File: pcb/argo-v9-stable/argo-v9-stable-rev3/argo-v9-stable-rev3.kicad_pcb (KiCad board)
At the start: 2 copper layers, 94.8 x 67.2 mm, 91 parts, among them IC1 MP2672GD, J1 Sparkfun_NEO-N9M-SMA, J2 USB4125-GF-A, J3 LED_power_button_RGB_LED, K1 PRL3-5V-DC-1A, Q2 BSD840N, SW1 POW, U1 orange_pi_zero_2w_2GB, U2 MAX11612, U3 CH221K, U5 SHT45-ADB1B, U6 RA-01, U7 TXS0102DCT

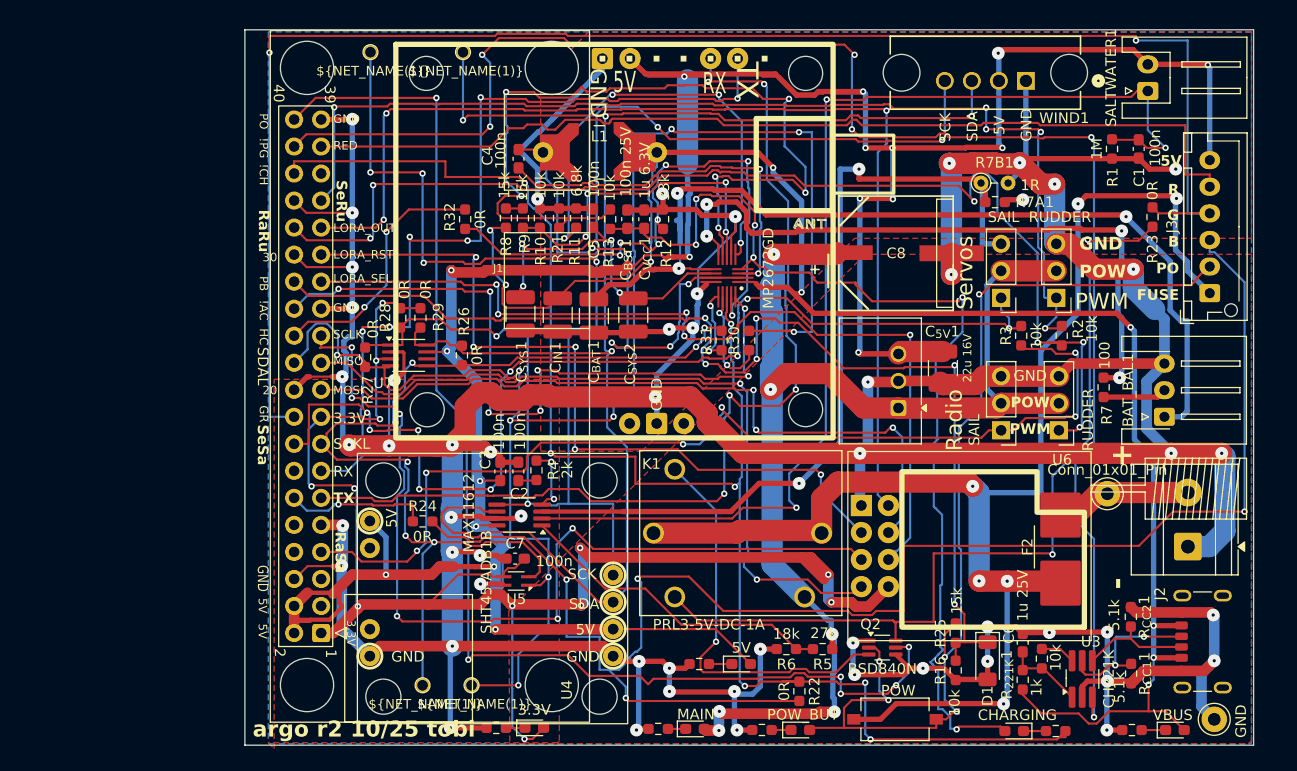
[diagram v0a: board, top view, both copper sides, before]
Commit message: argo pcb rev3 almost complete
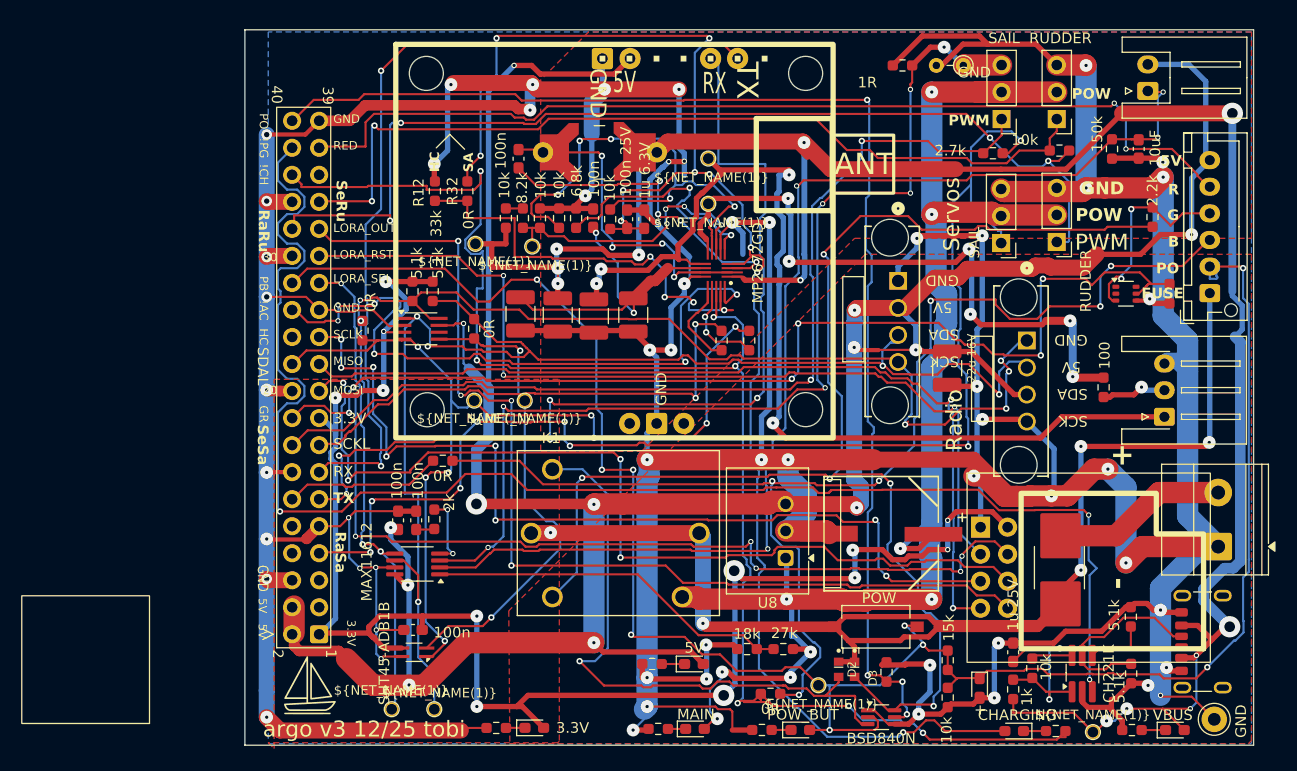
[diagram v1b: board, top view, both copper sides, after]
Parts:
- removed 5VREG1: Traco TSR1-2450E, Converter_DCDC:Converter_DCDC_TRACO_TSR1-xxxxE_THT
- removed BAT2: Conn_01x01_Pin, Connector_Pin:Pin_D1.0mm_L10.0mm_LooseFit
- added D2: TS4148_RCG, Argo footprint Library:DIO_TS4148_RCG, F.Cu at (113.0, 88.5)
- added D3: TS4148_RCG, Argo footprint Library:DIO_TS4148_RCG, F.Cu at (114.5, 88.5)
- added G***: LOGO, Argo footprint Library:argo-sailboat-icon, F.Cu at (63.2, 90.0)
- added Q1: BSD840N, Package_TO_SOT_SMD:SOT-363_SC-70-6, F.Cu at (140.0, 53.2)
- added R33: 10k, Resistor_SMD:R_0603_1608Metric_Pad0.98x0.95mm_HandSolder, F.Cu at (117.5, 88.8)
- added R34: 10k, Resistor_SMD:R_0603_1608Metric_Pad0.98x0.95mm_HandSolder, F.Cu at (144.1, 53.2)
- added TP10: TestPoint_Probe_autonamed, Argo footprint Library:TestPoint_scope_probe_autonamed, F.Cu at (84.2, 48.8)
- added TP11: TestPoint_Probe_autonamed, Argo footprint Library:TestPoint_scope_probe_autonamed, F.Cu at (136.9, 94.4)
- added TP5: TestPoint_Probe_autonamed, Argo footprint Library:TestPoint_scope_probe_autonamed, F.Cu at (78.9, 48.5)
- added TP6: TestPoint_Probe_autonamed, Argo footprint Library:TestPoint_scope_probe_autonamed, F.Cu at (111.1, 90.0)
- added TP8: TestPoint_Probe_autonamed, Argo footprint Library:TestPoint_scope_probe_autonamed, F.Cu at (100.8, 44.8)
- added TP9: TestPoint_Probe_autonamed, Argo footprint Library:TestPoint_scope_probe_autonamed, F.Cu at (100.8, 40.5)
- added U8: TSR_1-2450, Argo footprint Library:Converter_DCDC_TRACO_TSR1-xxxxE_THT, F.Cu at (108.0, 78.0)
- C1: value 100n -> 10uF
- D1: footprint Diode_SMD:D_MiniMELF -> Argo footprint Library:D_0603_1608Metric_hand_solder
- J3: footprint Connector_JST:JST_XH_B6B-XH-AM_1x06_P2.50mm_Vertical -> Argo footprint Library:JST_XH_B6B-XH-AM_1x06_P2.50mm_Vertical
- K1: footprint PRL3-5V-DC-1A:RELAY_PRL3-5V-DC-1A -> Argo footprint Library:RELAY_PRL3-5V-DC-1A
- Q2: footprint Package_TO_SOT_SMD:SOT-363_SC-70-6 -> Argo footprint Library:SOT-363_SC-70-6-handsolder
- R1: value 1M -> 150k
- R19: value 0R -> 1k
- R23: value 0R -> 2.2k
- R28, R29: value 0R -> 5.1k
- R3: value 10k -> 2.7k
- R8: value 15k -> 10k
- R9: value 15k -> 8.2k
- TP1: value SDA -> TestPoint_Probe_autonamed; footprint Argo footprint Library:TestPoint_scope_probe -> Argo footprint Library:TestPoint_scope_probe_autonamed
- TP2: value SCK -> TestPoint_Probe_autonamed; footprint Argo footprint Library:TestPoint_scope_probe -> Argo footprint Library:TestPoint_scope_probe_autonamed
- TP3: value SDAL -> TestPoint_Probe_autonamed; footprint Argo footprint Library:TestPoint_scope_probe -> Argo footprint Library:TestPoint_scope_probe_autonamed
- TP4: value SCKL -> TestPoint_Probe_autonamed; footprint Argo footprint Library:TestPoint_scope_probe -> Argo footprint Library:TestPoint_scope_probe_autonamed
- U1: footprint orangepi-zero:orange_pi_zero_2w -> Argo footprint Library:orange_pi_zero_2w_butted
- U4: footprint sparkfun:Sparkfun_IMU_ICM-20948 -> Argo footprint Library:I2C_header
- U5: footprint Sensor_Humidity:Sensirion_DFN-4_1.5x1.5mm_P0.8mm_SHT4x_NoCentralPad -> Argo footprint Library:Sensirion_DFN-4_1.5x1.5mm_P0.8mm_SHT4x_NoCentralPad-handsolder
- moved TP1 62.1 mm to (71.0, 92.2)
- moved TP2 62.0 mm to (75.0, 92.2)
- moved U4 47.7 mm to (118.6, 52.0)
- moved TP3 27.2 mm to (83.5, 63.2)
- moved TP4 27.2 mm to (78.8, 63.2)
- moved C8 26.4 mm to (117.0, 75.8), turned to 180 degrees
- moved WIND1 24.4 mm to (130.7, 57.6), turned to 90 degrees
- moved U1 23.4 mm to (66.2, 93.7)
- moved R12 21.6 mm to (75.1, 43.6)
- moved U6 19.9 mm to (129.9, 86.8), turned to 0 degrees
- moved RADIO_RUDDER1 17.7 mm to (133.5, 48.3)
- moved RADIO_SAIL1 17.6 mm to (128.3, 48.4)
- moved R2 17.4 mm to (133.8, 39.8), turned to 180 degrees
- moved R3 17.4 mm to (127.5, 40.0), turned to 180 degrees
- moved SERVO_RUDDER1 16.8 mm to (133.5, 36.8)
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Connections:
- J3 pad 2: /POW_ON -> /POW_BUT
- POW_BUT1 pad 2: /POW_ON -> /POW_BUT
- Q2 pad 2: /POW_ON -> /POW_BUT
- R25 pad 2: /POW_ON -> /POW_BUT
- R32 pad 2: /HOST_CTL -> /VCC_LDO
- SW1 pad 2: /POW_ON -> /POW_BUT
- TP1 pad 1: /SDA -> /SCK
- TP2 pad 1: /SCK -> /SDA
- TP3 pad 1: /SDAL -> /SCKL
- TP4 pad 1: /SCKL -> /SDAL
- U1 pad 18: /GREEN -> /PH4
- U6 pad 5: +3.3V -> /LORA_OUT
- U6 pad 6: /!LORA_SEL -> /MOSI
- U6 pad 7: /MOSI -> /!LORA_SEL
- U6 pad 8: /LORA_OUT -> +3.3V
- U7 pad 1: /SCK -> /SDA
- U7 pad 8: /SDA -> /SCK
- WIND1 pad 1: GND -> /SCK
- WIND1 pad 2: 5V -> /SDA
- WIND1 pad 3: /SDA -> 5V
- WIND1 pad 4: /SCK -> GND
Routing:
- net GND: track 591.5 -> 726.4 mm, vias 55 -> 58
- net /GREEN: track 148.9 -> 19.1 mm
- net /PH4: track 0.00 -> 102.4 mm, vias 0 -> 6
- net /POW_ON: track 95.2 -> 0.00 mm, vias 5 -> 0
- net /POW_BUT: track 106.8 -> 190.1 mm, vias 6 -> 9
- net /VBUS: track 162.1 -> 245.1 mm, vias 9 -> 12
- net /SDAL: track 152.2 -> 87.9 mm, vias 9 -> 8
- net 5V: track 339.7 -> 280.1 mm, vias 18 -> 13
- net /PSR: track 82.6 -> 130.5 mm, vias 2 -> 5
- net /SCK: track 173.4 -> 125.8 mm
- net /VCC_LDO: track 97.2 -> 144.4 mm, vias 6 -> 10
- net Net-(IC1-NTC): track 81.3 -> 46.5 mm, vias 6 -> 5
- net /BLUE: track 151.4 -> 117.9 mm, vias 4 -> 6
- net /MAIN: track 115.9 -> 146.4 mm, vias 6 -> 9
- net /SDA: track 153.2 -> 128.7 mm, vias 4 -> 5
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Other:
- board text added: "SA"
- board text added: "argo v3 12/25 tobi"
- board text removed: "argo r2 10/25 tobi"
